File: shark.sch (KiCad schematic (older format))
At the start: 252 parts, among them J1 USB_C_Receptacle, Q1 AO4406AL, SW1 MXSwitch, SW10 MXSwitch, SW11 MXSwitch, SW12 MXSwitch, SW13 MXSwitch, SW14 MXSwitch, SW15 MXSwitch, SW16 MXSwitch, SW17 MXSwitch, SW18 MXSwitch, SW19 MXSwitch, SW2 MXSwitch, SW20 MXSwitch, SW21 MXSwitch, SW22 MXSwitch, SW23 MXSwitch, SW24 MXSwitch, SW25 MXSwitch, SW26 MXSwitch, SW27 MXSwitch, SW28 MXSwitch, SW29 MXSwitch, SW3 MXSwitch, SW30 MXSwitch, SW31 MXSwitch, SW32 MXSwitch, SW33 MXSwitch, SW34 MXSwitch, SW35 MXSwitch, SW36 MXSwitch, SW37 MXSwitch, SW38 MXSwitch, SW39 MXSwitch, SW4 MXSwitch, SW40 MXSwitch, SW41 MXSwitch, SW42 MXSwitch, SW43 MXSwitch, SW44 MXSwitch, SW45 MXSwitch, SW46 MXSwitch, SW47 MXSwitch, SW48 MXSwitch, SW49 MXSwitch, SW5 MXSwitch, SW50 MXSwitch, SW51 MXSwitch, SW6 MXSwitch, SW7 MXSwitch, SW8 MXSwitch, SW9 MXSwitch, U1 STM32F303CCT7, U2 MCP1700-3302E_SOT23, Y1 8MHz

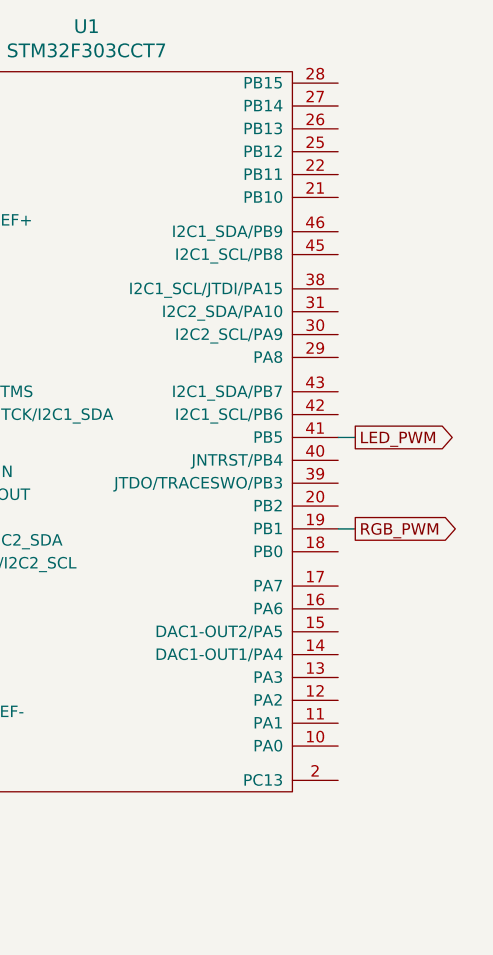
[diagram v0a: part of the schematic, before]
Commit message: Continued routing
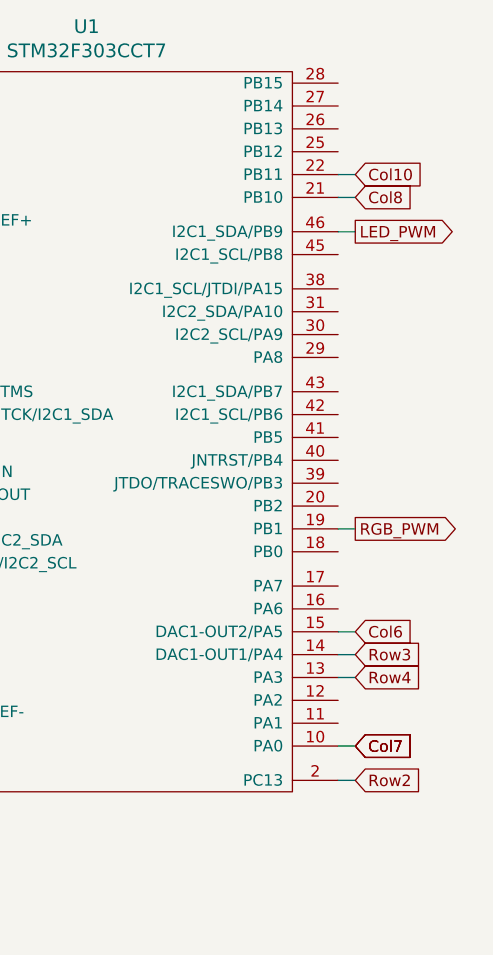
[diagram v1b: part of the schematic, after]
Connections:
- net Col10: now also U1.22 (PB11)
- net Col6: now also U1.15 (DAC1-OUT2/PA5)
- net Col7: now also U1.10 (PA0)
- net Col8: now also U1.21 (PB10)
- net LED_PWM: now also U1.46 (I2C1_SDA/PB9); no longer U1.41 (PB5)
- net Row2: now also U1.2 (PC13)
- net Row3: now also U1.14 (DAC1-OUT1/PA4)
- net Row4: now also U1.13 (PA3)
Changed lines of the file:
@@
 Wire Wire Line
 	3475 10800 4125 10800
-Text GLabel 15375 7775 2    50   Output ~ 0
+Text GLabel 15375 6875 2    50   Output ~ 0
 LED_PWM
 Wire Wire Line
-	15375 7775 15300 7775
+	15375 6875 15300 6875
 Text GLabel 2825 9100 1    50   Input ~ 0
 5V
@@
 Text GLabel 5875 8750 0    50   Input ~ 0
 3.3V
+Text GLabel 15375 9125 2    50   Input ~ 0
+Col7
+Wire Wire Line
+	15375 9125 15300 9125
+Text GLabel 15375 8725 2    50   Input ~ 0
+Row3
+Text GLabel 15375 9275 2    50   Input ~ 0
+Row2
+Wire Wire Line
+	15375 9275 15300 9275
+Text GLabel 15375 8825 2    50   Input ~ 0
+Row4
+Wire Wire Line
+	15375 8825 15300 8825
+Wire Wire Line
+	15375 8725 15300 8725
+Text GLabel 15375 9125 2    50   Input ~ 0
+Col7
+Text GLabel 15375 8625 2    50   Input ~ 0
+Col6
+Wire Wire Line
+	15375 8625 15300 8625
+Text GLabel 15375 6625 2    50   Input ~ 0
+Col10
+Wire Wire Line
+	15375 6625 15300 6625
+Text GLabel 15375 6725 2    50   Input ~ 0
+Col8
+Wire Wire Line
+	15375 6725 15300 6725
 $EndSCHEMATC
